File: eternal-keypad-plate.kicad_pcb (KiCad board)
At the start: 2 copper layers, 163.5 x 95.3 mm, 42 parts

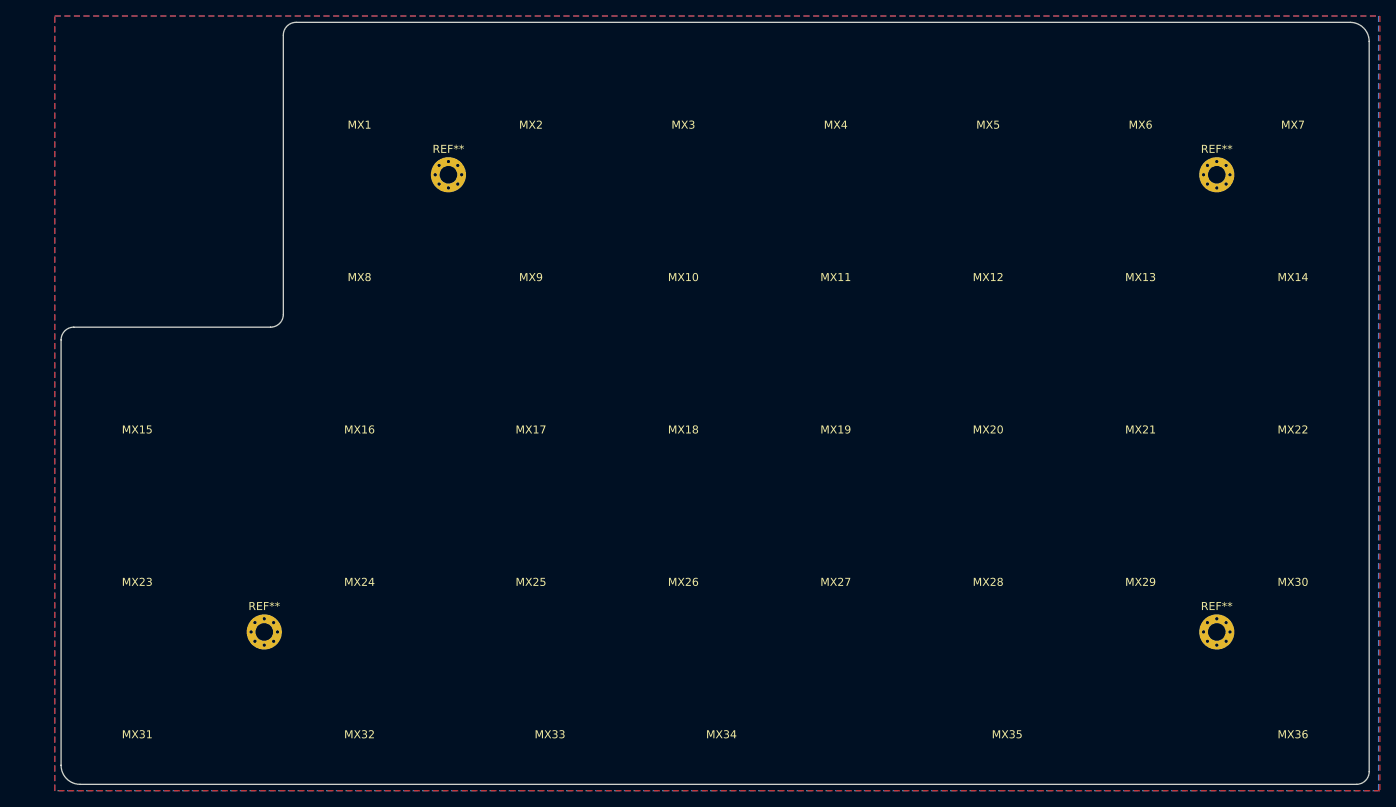
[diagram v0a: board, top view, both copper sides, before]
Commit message: Final adjustments and case patterns
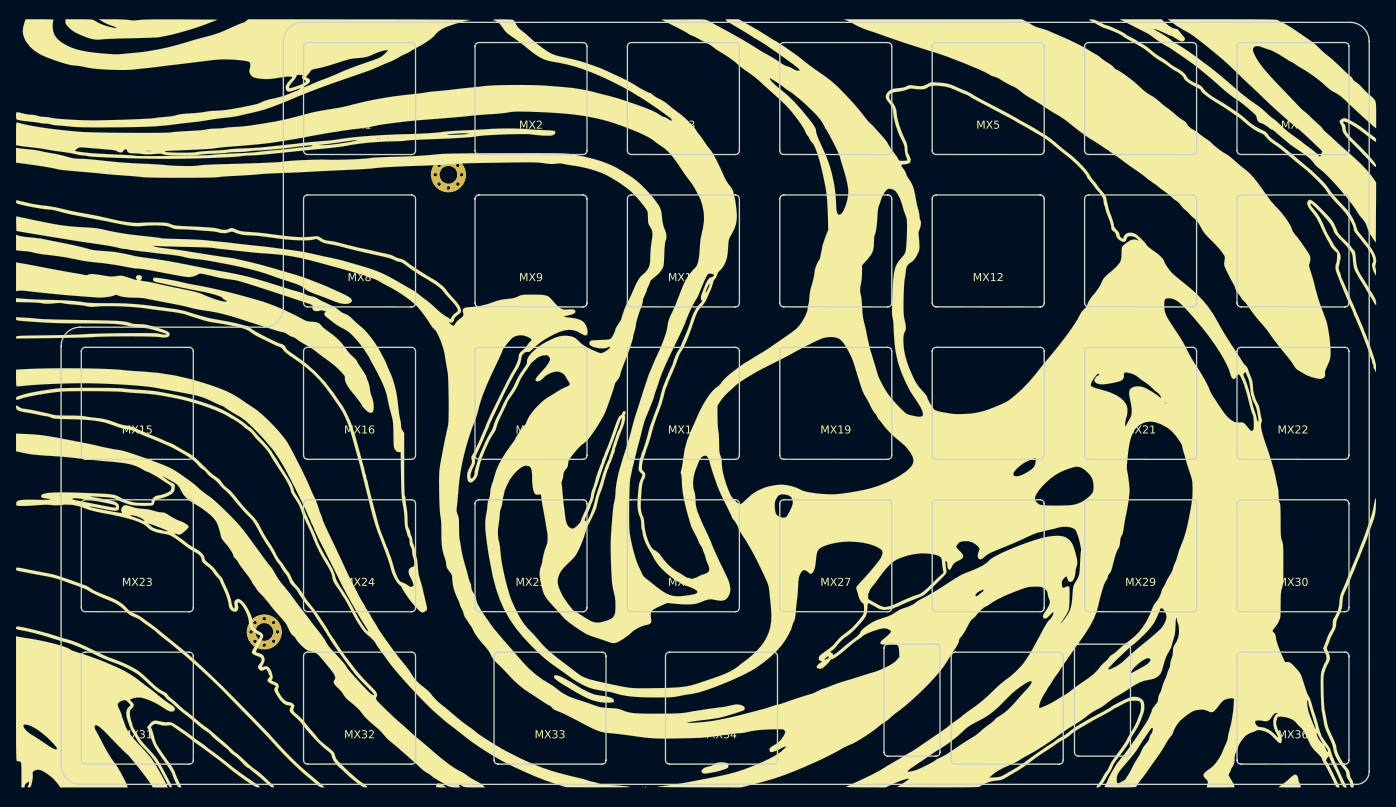
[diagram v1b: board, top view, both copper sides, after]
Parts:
- removed the REF** at (172.2, 125.4)
- added G***: LOGO, Symbol:paint-swirl, B.Cu at (132.6, 87.3)
- added G***: LOGO, Symbol:paint-swirl, F.Cu at (133.3, 87.3)
- added REF**: MX275, acheron_MX_PlateSlots:MX275, F.Cu at (172.2, 125.4)
- MX1, MX10, MX11, MX12, MX13, MX14, MX15, MX16, MX17, MX18, MX19, MX2, MX20, MX21, MX22, MX23, MX24, MX25, MX26, MX27, MX28, MX29, MX3, MX30, MX31, MX32, MX33, MX34, MX35, MX36, MX4, MX5, MX6, MX7, MX8, MX9: footprint Keebio-Parts:MX_Switch_Cutout -> acheron_MX_PlateSlots:MX100
- REF** (x4): value MountingHole_2.2mm_M2_Pad_Via -> MountingHole_4.6mm_Pad_Via
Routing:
- removed copper zone on B.Cu, net GND
- removed copper zone on F.Cu, net GND
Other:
- outline, holes or cut-outs redrawn
